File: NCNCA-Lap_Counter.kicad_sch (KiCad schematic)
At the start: 1 part

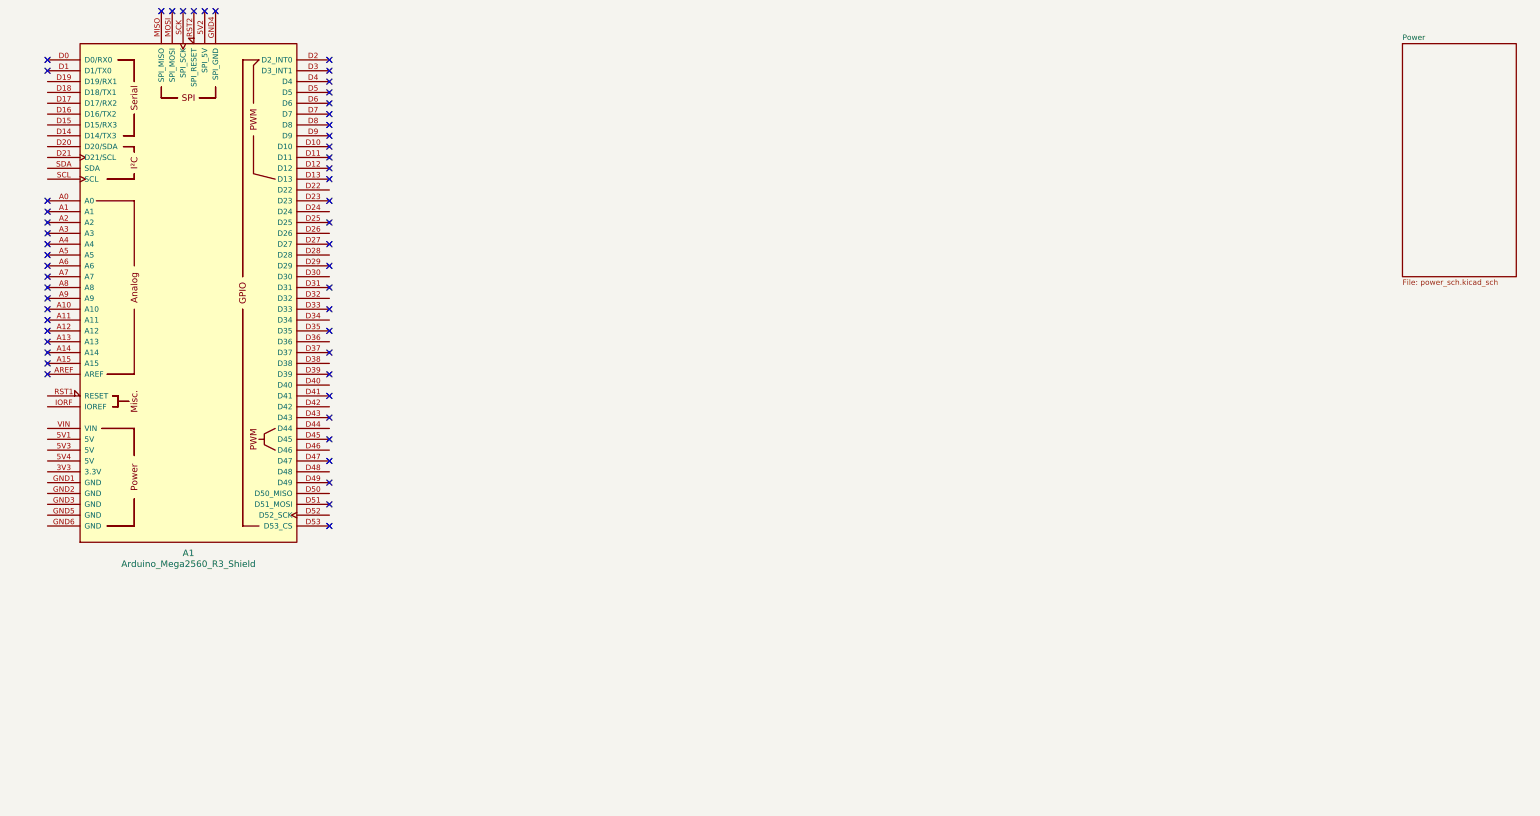
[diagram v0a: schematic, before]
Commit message: Schematic in state of received unit.  Will branch from here.
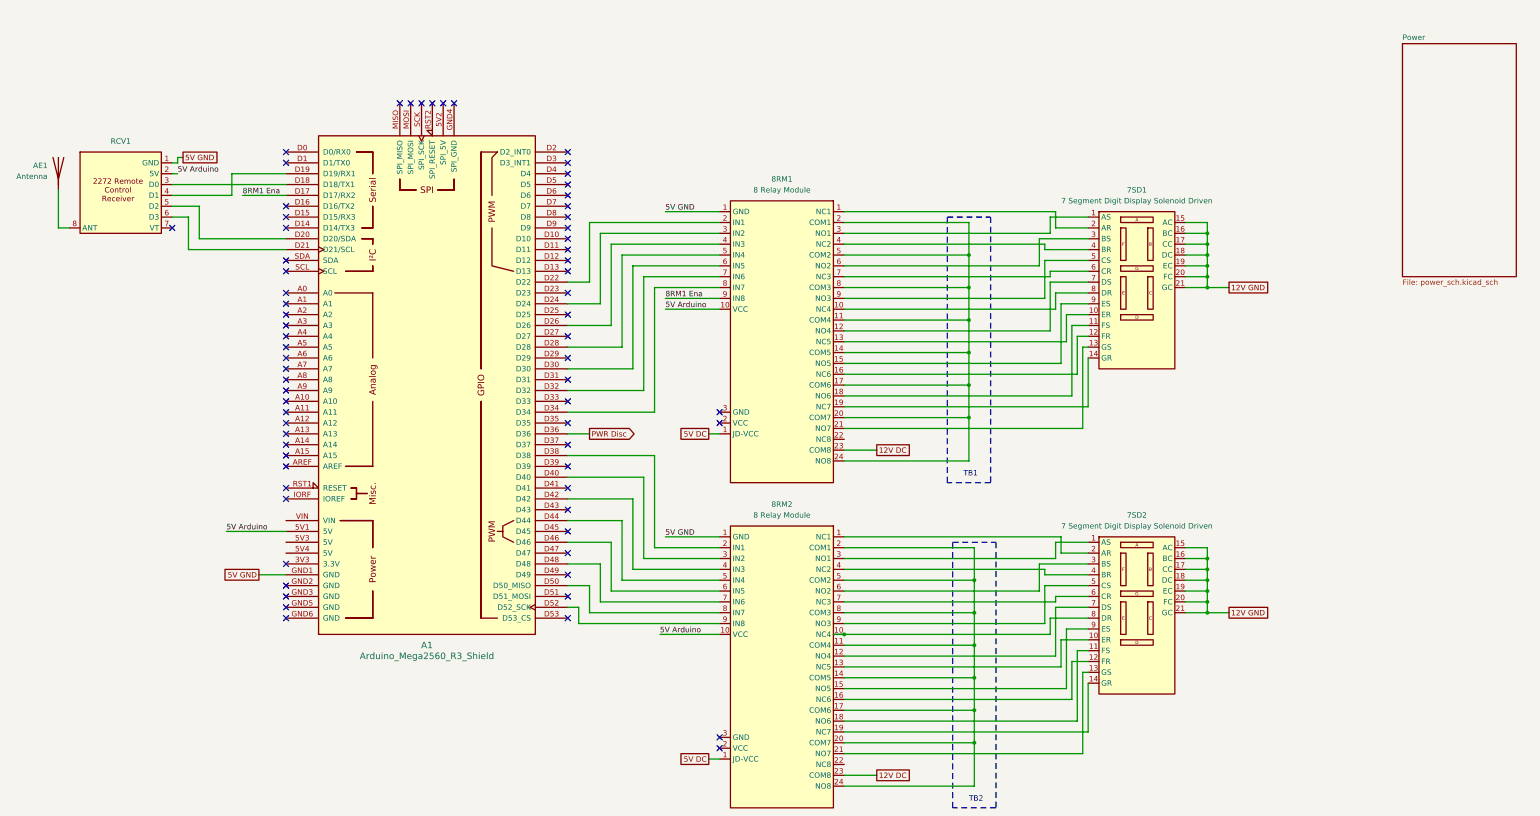
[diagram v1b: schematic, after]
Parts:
- added 7SD1, 7SD2: 7 Segment Digit Display Solenoid Driven, symbol Project Library:7_Segment_Solenoid
- added 8RM1, 8RM2: 8 Relay Module, symbol Project Library:8_Relay_Module
- added AE1: Antenna, symbol Device:Antenna
- added RCV1: ~, symbol Project Library:Marstech_2272_Receiver
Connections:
- net 5V Arduino: now reaches A1.5V1 (5V)
- net 5V Arduino: now also 8RM1.10 (VCC), 8RM2.10 (VCC), RCV1.2 (5V)
- net 8RM1 Ena: now reaches A1.D17 (D17/RX2)
- net 8RM1 Ena: now also 8RM1.9 (NO3)
- net at A1.D18 (D18/TX1): now also RCV1.3 (D0)
- net at A1.D19 (D19/RX1): now also RCV1.4 (D1)
- net at A1.D20 (D20/SDA): now also RCV1.5 (D2)
- net at A1.D21 (D21/SCL): now also RCV1.6 (D3)
- net at A1.D22: now also 8RM1.2 (VCC)
- net at A1.D24: now also 8RM1.3 (NO1)
- net at A1.D26: now also 8RM1.4 (NC2)
- net at A1.D28: now also 8RM1.5 (IN4)
- net at A1.D30: now also 8RM1.6 (NO2)
- net at A1.D32: now also 8RM1.7 (NC3)
- net at A1.D34: now also 8RM1.8 (IN7)
- net PWR Disc: now reaches A1.D36
- net at A1.D38: now also 8RM2.2 (VCC)
- net at A1.D40: now also 8RM2.3 (NO1)
- net at A1.D42: now also 8RM2.4 (NC2)
- net at A1.D44: now also 8RM2.5 (IN4)
- net at A1.D46: now also 8RM2.6 (NO2)
- net at A1.D48: now also 8RM2.7 (NC3)
- net at A1.D50 (D50_MISO): now also 8RM2.8 (IN7)
- net at A1.D52 (D52_SCK): now also 8RM2.9 (NO3)
- net 5V GND: now reaches A1.GND1 (GND)
- net 5V GND: now also 8RM1.1 (NC1), 8RM2.1 (NC1), RCV1.1 (GND)
- new net: 7SD1.1 (AS), 8RM1.3 (NO1)
- new net: 7SD1.10 (ER), 8RM1.13 (NC5)
- new net: 7SD1.11 (FS), 8RM1.18 (NO6)
- new net: 7SD1.12 (FR), 8RM1.16 (NC6)
- new net: 7SD1.13 (GS), 8RM1.21 (NO7)
- new net: 7SD1.14 (GR), 8RM1.19 (NC7)
- new net: 7SD1.2 (AR), 8RM1.1 (NC1)
- new net: 7SD1.3 (BS), 8RM1.6 (NO2)
- new net: 7SD1.4 (BR), 8RM1.4 (NC2)
- new net: 7SD1.5 (CS), 8RM1.9 (NO3)
- new net: 7SD1.6 (CR), 8RM1.7 (NC3)
- new net: 7SD1.7 (DS), 8RM1.12 (NO4)
- new net: 7SD1.8 (DR), 8RM1.10 (VCC)
- new net: 7SD1.9 (ES), 8RM1.15 (NO5)
- new net: 7SD2.1 (AS), 8RM2.3 (NO1)
- new net: 7SD2.10 (ER), 8RM2.13 (NC5)
- new net: 7SD2.11 (FS), 8RM2.18 (NO6)
- new net: 7SD2.12 (FR), 8RM2.16 (NC6)
- new net: 7SD2.13 (GS), 8RM2.21 (NO7)
- new net: 7SD2.14 (GR), 8RM2.19 (NC7)
- new net: 7SD2.2 (AR), 8RM2.1 (NC1)
- new net: 7SD2.3 (BS), 8RM2.6 (NO2)
- new net: 7SD2.4 (BR), 8RM2.4 (NC2)
- new net: 7SD2.5 (CS), 8RM2.9 (NO3)
- new net: 7SD2.6 (CR), 8RM2.7 (NC3)
- new net: 7SD2.7 (DS), 8RM2.12 (NO4)
- new net: 7SD2.8 (DR), 8RM2.10 (VCC)
- new net: 7SD2.9 (ES), 8RM2.15 (NO5)
- new net: 8RM2.11 (COM4), 8RM2.14 (COM5), 8RM2.17 (COM6), 8RM2.2 (VCC), 8RM2.20 (COM7), 8RM2.24 (NO8), 8RM2.5 (IN4), 8RM2.8 (IN7)
- new net: AE1.1 (A), RCV1.8 (ANT)
- new net: 8RM1.11 (COM4), 8RM1.14 (COM5), 8RM1.17 (COM6), 8RM1.2 (VCC), 8RM1.20 (COM7), 8RM1.24 (NO8), 8RM1.5 (IN4), 8RM1.8 (IN7)
- new net 12V DC: 8RM1.23 (COM8), 8RM2.23 (COM8)
- new net 12V GND: 7SD1.15 (AC), 7SD1.16 (BC), 7SD1.17 (CC), 7SD1.18 (DC), 7SD1.19 (EC), 7SD1.20 (FC), 7SD1.21 (GC), 7SD2.15 (AC), 7SD2.16 (BC), 7SD2.17 (CC), 7SD2.18 (DC), 7SD2.19 (EC), 7SD2.20 (FC), 7SD2.21 (GC)
- new net 5V DC: 8RM1.1 (NC1), 8RM2.1 (NC1)
- no-connect marks 53 -> 70
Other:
- note added: "TB1"
- note added: "TB2"
- moved on the sheet: A1
